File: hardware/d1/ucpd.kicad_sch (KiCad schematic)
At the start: 3 parts, among them U4 TCPP03-M20, U5 TCPP03-M20

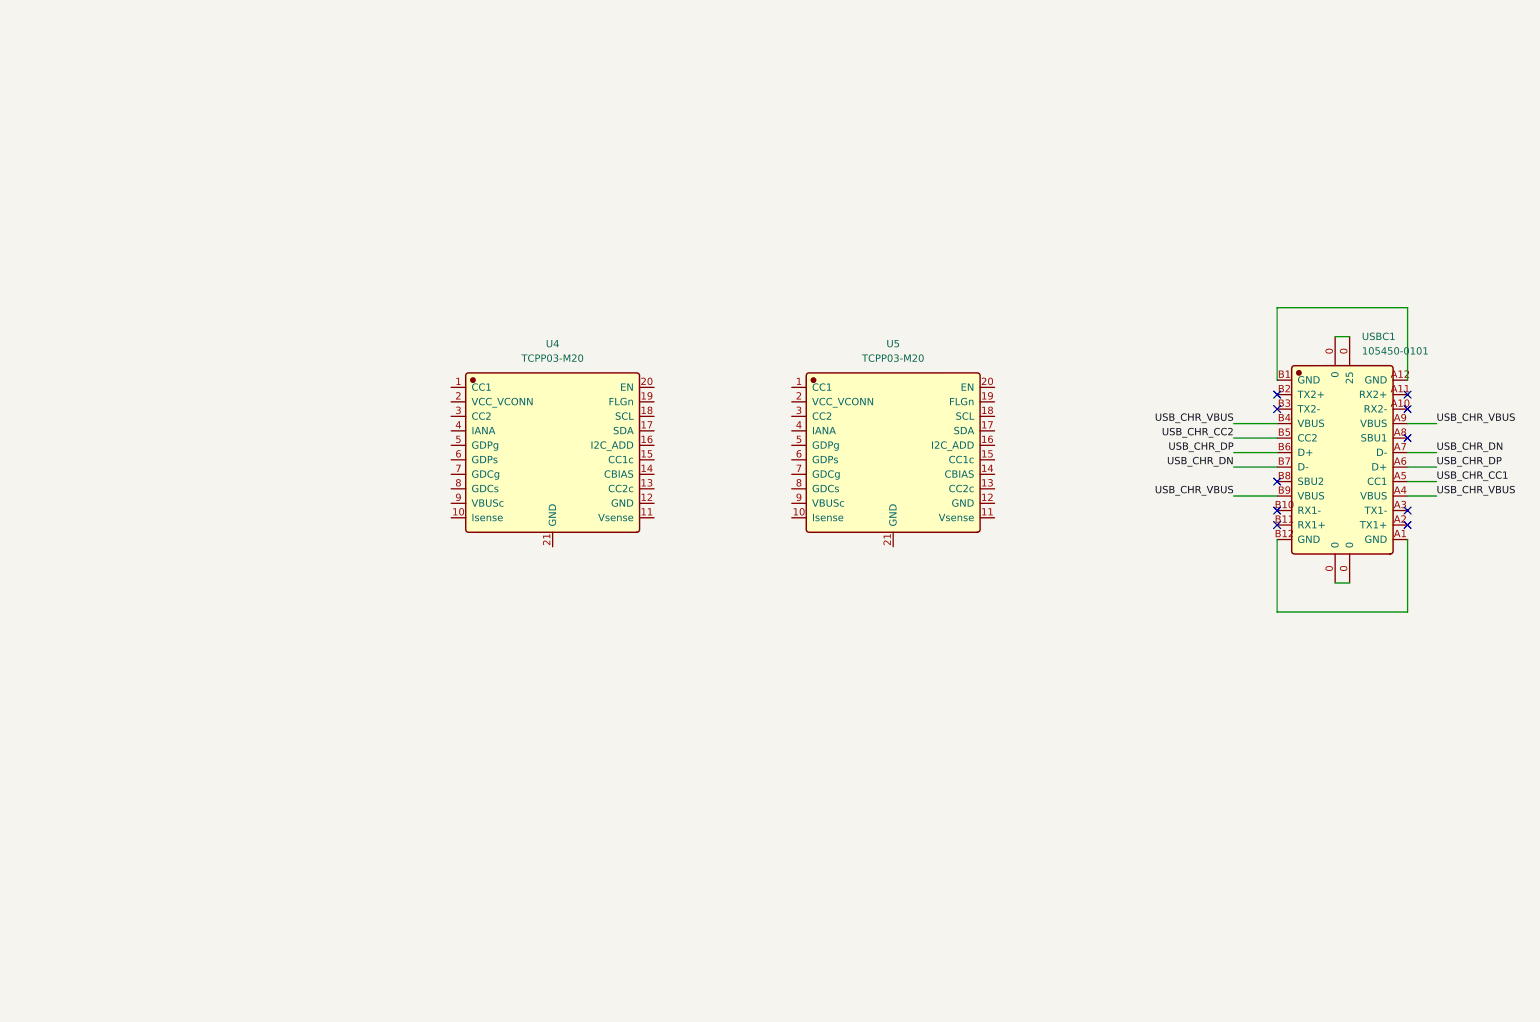
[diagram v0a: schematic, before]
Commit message: Pre-finalize sch
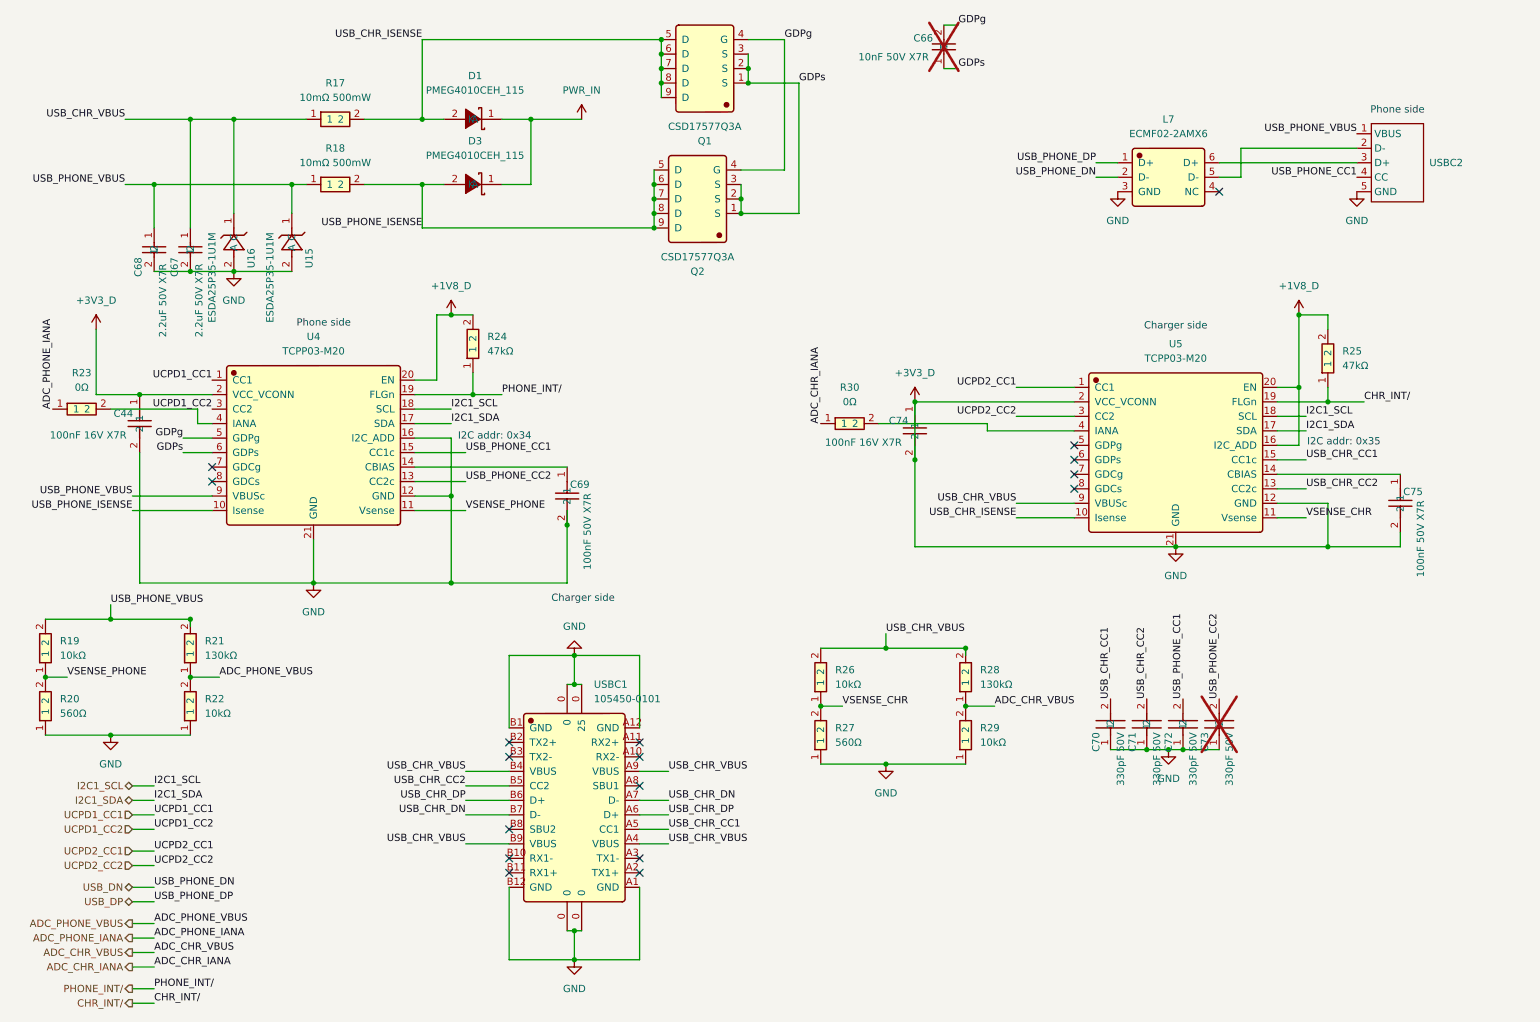
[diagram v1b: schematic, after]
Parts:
- added C44, C74: 100nF 16V X7R, JLCImport:CL05B104KO5NNNC, symbol JLCImport:CL05B104KO5NNNC
- added C66: 10nF 50V X7R, Capacitor_SMD:C_0402_1005Metric, symbol JLCImport:CL05B103KB5NNNC
- added C67, C68: 2.2uF 50V X7R, JLCImport:CC0805KKX7R9BB225, symbol JLCImport:CC0805KKX7R9BB225
- added C69, C75: 100nF 50V X7R, JLCImport:CL05B104KB54PNC, symbol JLCImport:CL05B104KB54PNC
- added C70, C71, C72, C73: 330pF 50V, Capacitor_SMD:C_0402_1005Metric, symbol JLCImport:CL05C331JB5NNNC
- added D1, D3: PMEG4010CEH_115, Diode_SMD:D_SOD-110, symbol JLCImport:PMEG4010CEH_115
- added L7: ECMF02-2AMX6, JLCImport:ECMF02-2AMX6, symbol JLCImport:ECMF02-2AMX6
- added Q1, Q2: CSD17577Q3A, JLCImport:CSD17577Q3A, symbol JLCImport:CSD17577Q3A
- added R17, R18: 10mΩ 500mW, Resistor_SMD:R_0805_2012Metric, symbol JLCImport:ERJ6BWFR010V
- added R19, R22, R26, R29: 10kΩ, Resistor_SMD:R_0402_1005Metric, symbol JLCImport:0402WGF1002TCE
- added R20, R27: 560Ω, Resistor_SMD:R_0402_1005Metric, symbol JLCImport:0402WGF5600TCE
- added R21, R28: 130kΩ, Resistor_SMD:R_0402_1005Metric, symbol JLCImport:RC0402FR-07130KL
- added R23, R30: 0Ω, Resistor_SMD:R_0402_1005Metric, symbol JLCImport:RC0402FR-070RL
- added R24, R25: 47kΩ, Resistor_SMD:R_0402_1005Metric, symbol JLCImport:0402WGF4702TCE
- added U15, U16: ESDA25P35-1U1M, JLCImport:ESDA25P35-1U1M_C19829649, symbol JLCImport:ESDA25P35-1U1M_C19829649
- added USBC2: (no value), JLCImport:USBC_EXT_5P, symbol JLCImport:USBC_5P_EXT
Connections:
- net USB_CHR_CC1: now also U5.15 (CC1c), C70.2
- net USB_CHR_CC2: now also U5.13 (CC2c), C71.2
- net USB_CHR_VBUS: now also U5.9 (VBUSc), C67.1, R17.1, R26.2, R28.2, U16.1 (C)
- net UCPD2_CC1: now reaches U5.1 (CC1)
- net USB_CHR_ISENSE: now reaches U5.10 (Isense)
- net USB_CHR_ISENSE: now also D1.2 (A), Q1.5 (D), Q1.6 (D), Q1.7 (D), Q1.8 (D), Q1.9 (D), R17.2
- net VSENSE_CHR: now reaches U5.11 (Vsense)
- net VSENSE_CHR: now also R26.1, R27.2
- net +3V3_D: now reaches U5.12 (GND)
- net +3V3_D: now also U4.12 (GND), U4.16 (I2C_ADD), U4.2 (VCC_VCONN), U4.21 (GND), U5.2 (VCC_VCONN), U5.21 (GND), USBC1.0, USBC1.A1 (GND), USBC1.A12 (GND), USBC1.B1 (GND), USBC1.B12 (GND), C44.1, C44.2, C67.2, C68.2, C69.2, C70.1, C71.1, C72.1, C73.1, C74.1, C74.2, C75.2, L7.3 (GND), R20.1, R22.1, R27.1, R29.1, U15.2 (A), U16.2 (A), USBC2.5 (GND)
- net at U5.14 (CBIAS): now also C75.1
- net +1V8_D: now reaches U5.16 (I2C_ADD)
- net +1V8_D: now also U4.20 (EN), U5.20 (EN), R24.2, R25.2
- net I2C1_SDA: now reaches U5.17 (SDA)
- net I2C1_SDA: now also U4.17 (SDA)
- net I2C1_SCL: now reaches U5.18 (SCL)
- net I2C1_SCL: now also U4.18 (SCL)
- net CHR_INT/: now reaches U5.19 (FLGn)
- net CHR_INT/: now also R25.1
- net UCPD2_CC2: now reaches U5.3 (CC2)
- net at U5.4 (IANA): now also R30.2
- net UCPD1_CC1: now reaches U4.1 (CC1)
- net USB_PHONE_ISENSE: now reaches U4.10 (Isense)
- net USB_PHONE_ISENSE: now also D3.2 (A), Q2.5 (D), Q2.6 (D), Q2.7 (D), Q2.8 (D), Q2.9 (D), R18.2
- net VSENSE_PHONE: now reaches U4.11 (Vsense)
- net VSENSE_PHONE: now also R19.1, R20.2
- net USB_PHONE_CC2: now reaches U4.13 (CC2c)
- net USB_PHONE_CC2: now also C73.2
- net at U4.14 (CBIAS): now also C69.1
- net USB_PHONE_CC1: now reaches U4.15 (CC1c)
- net USB_PHONE_CC1: now also C72.2, USBC2.4 (CC)
- net PHONE_INT/: now reaches U4.19 (FLGn)
- net PHONE_INT/: now also R24.1
- net UCPD1_CC2: now reaches U4.3 (CC2)
- net at U4.4 (IANA): now also R23.2
- net GDPg: now reaches U4.5 (GDPg)
- net GDPg: now also C66.2, Q1.4 (G), Q2.4 (G)
- net GDPs: now reaches U4.6 (GDPs)
- net GDPs: now also C66.1, Q1.1 (S), Q1.2 (S), Q1.3 (S), Q2.1 (S), Q2.2 (S), Q2.3 (S)
- net USB_PHONE_VBUS: now reaches U4.9 (VBUSc)
- net USB_PHONE_VBUS: now also C68.1, R18.1, R19.2, R21.2, U15.1 (C), USBC2.1 (VBUS)
- new net: L7.5 (D-), USBC2.2 (D-)
- new net: L7.6 (D+), USBC2.3 (D+)
- new net ADC_CHR_IANA: R30.1
- new net ADC_CHR_VBUS: R28.1, R29.2
- new net ADC_PHONE_IANA: R23.1
- new net ADC_PHONE_VBUS: R21.1, R22.2
- new net PWR_IN: D1.1 (K), D3.1 (K)
- new net USB_DN: L7.2 (D-)
- new net USB_DP: L7.1 (D+)
- no-connect marks 10 -> 17
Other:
- note added: "Charger side"
- note added: "I2C addr: 0x34"
- note added: "I2C addr: 0x35"
- note added: "Phone side"
- moved on the sheet: U4, U5, USBC1

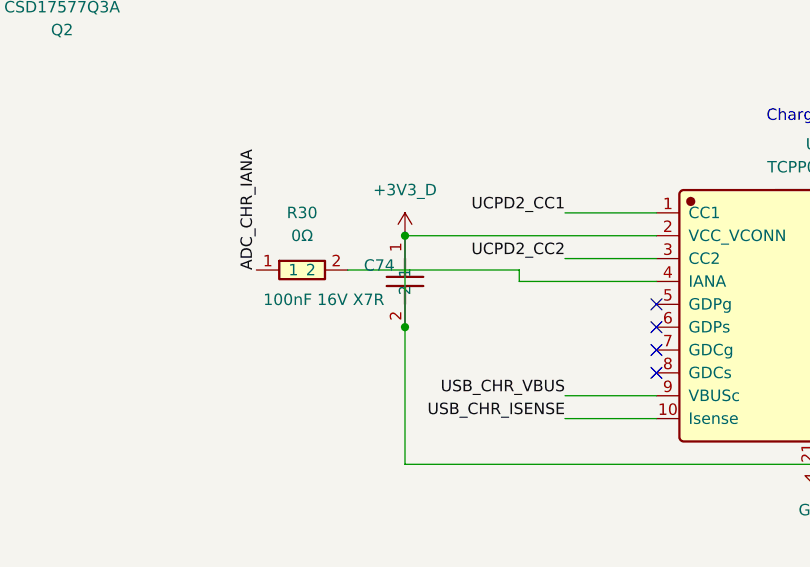
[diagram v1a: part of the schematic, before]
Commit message: Fix issue, add exti
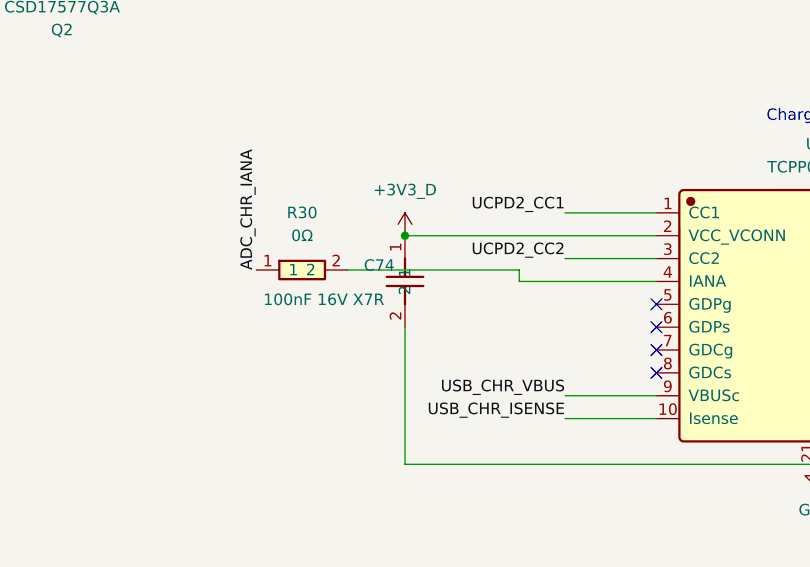
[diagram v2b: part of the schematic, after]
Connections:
- net +3V3_D: no longer C44.2, C67.2, C68.2, C69.2, C70.1, C71.1, C72.1, C73.1, C74.2, C75.2, L7.3 (GND), R20.1, R22.1, R27.1, R29.1, U15.2 (A), U16.2 (A), U4.12 (GND), U4.16 (I2C_ADD), U4.21 (GND), U5.12 (GND), U5.21 (GND), USBC1.0, USBC1.A1 (GND), USBC1.A12 (GND), USBC1.B1 (GND), USBC1.B12 (GND), USBC2.5 (GND)
- new net GND: C44.2, C67.2, C68.2, C69.2, C70.1, C71.1, C72.1, C73.1, C74.2, C75.2, L7.3 (GND), R20.1, R22.1, R27.1, R29.1, U15.2 (A), U16.2 (A), U4.12 (GND), U4.16 (I2C_ADD), U4.21 (GND), U5.12 (GND), U5.21 (GND), USBC1.0, USBC1.A1 (GND), USBC1.A12 (GND), USBC1.B1 (GND), USBC1.B12 (GND), USBC2.5 (GND)
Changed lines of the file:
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@@
-	)
-	(junction
-		(at 168.91 96.52)
-		(diameter 0)
-		(color 0 0 0 0)
 	)
 	(junction
@@
 		)
 		(stroke
-			(width 0)
-			(type default)
-		)
-	)
-	(wire
-		(pts
-			(xy 168.91 86.36) (xy 168.91 96.52)
-		)
-		(stroke
